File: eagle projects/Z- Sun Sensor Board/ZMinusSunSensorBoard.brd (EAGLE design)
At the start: 91 x 91 mm, 204 parts, among them J1 TE-1734829-2, U1 ADS7841E_2K5, U10 TSV991AILT, U11 TSV991AILT, U12 TSV991AILT, U13 ADS7841E_2K5, U14 TSV991AILT, U16 TSV991AILT, U17 TSV991AILT, U19 TSV991AILT, U2 ADS7841E_2K5, U21 TSV991AILT, U23 TSV991AILT, U25 ADS7841E_2K5, U26 TSV991AILT, U27 ADS7841E_2K5, U29 TSV991AILT, U3 TSV991AILT, U4 LM20BIM7X_NOPB, U5 LM20BIM7X_NOPB, U6 TSV991AILT, U8 TSV991AILT, U9 TSV991AILT

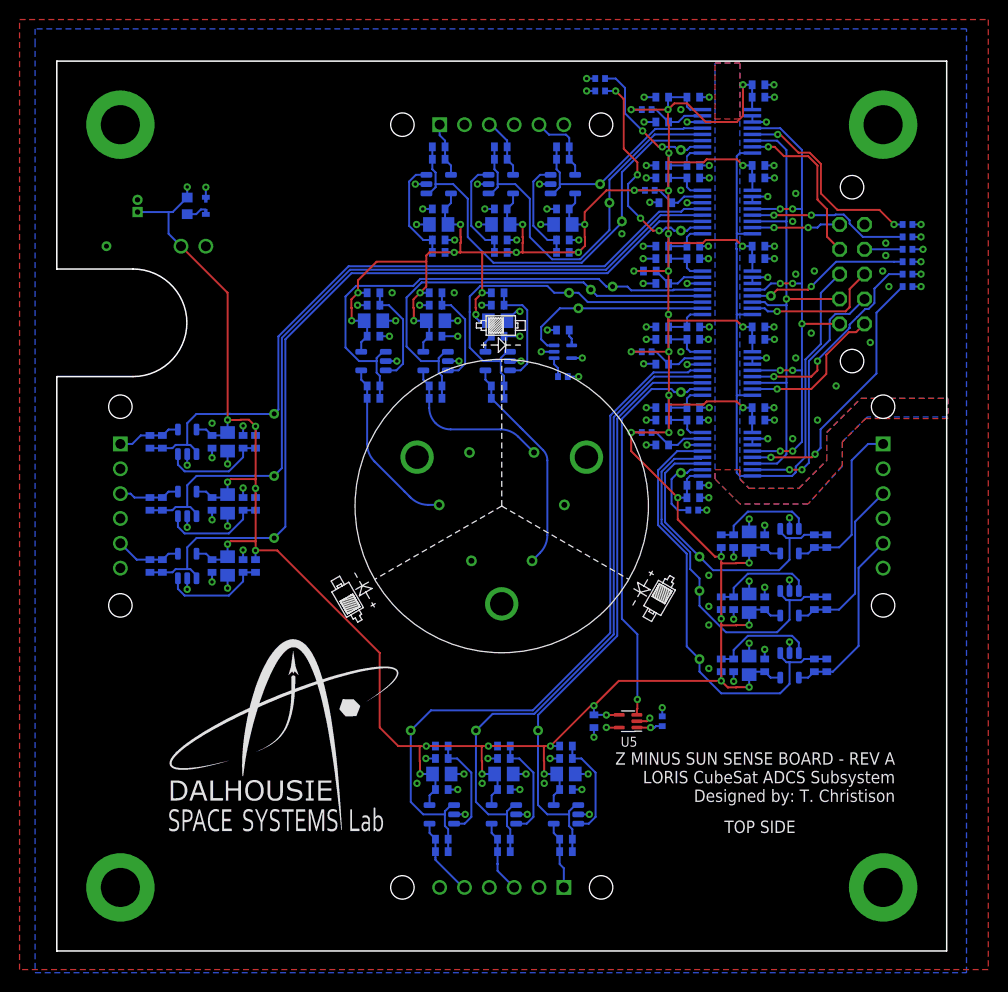
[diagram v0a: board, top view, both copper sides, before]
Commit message: I thinks its done
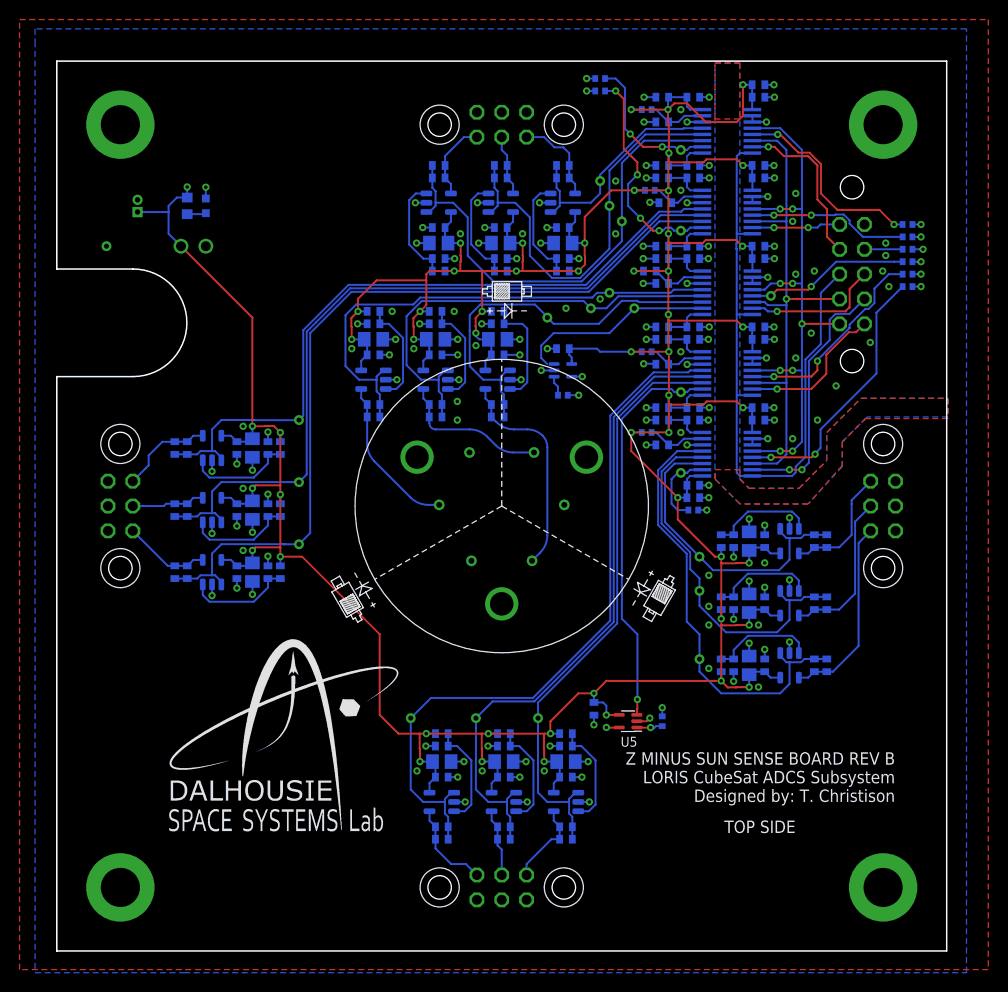
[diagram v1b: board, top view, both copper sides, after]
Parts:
- JP2, JP4, JP5, JP6: device my_library:1X06_MTG_HOLES -> my_library:2X03_MTG_HOLES
- LED1: device led:CHIPLED-0603-TTW -> led:CHIP-LED0603
- moved TP1 5.71 mm to (59.1, 65.7)
- moved U$3 3.55 mm to (46.0, 66.7)
- moved TP3 3.38 mm to (50.2, 64.8)
- moved C100 2.62 mm to (20.0, 38.7)
- moved C71 2.62 mm to (20.0, 51.4)
- moved C87 2.62 mm to (20.0, 45.1)
- moved R66 2.62 mm to (13.3, 51.4)
- moved R75 2.62 mm to (13.3, 45.1)
- moved R81 2.62 mm to (13.3, 38.7)
- moved TP23 2.62 mm to (24.8, 54.3)
- moved C101 2.62 mm to (18.4, 38.7)
- moved C103 2.62 mm to (12.1, 38.7)
- moved C82 2.62 mm to (18.4, 51.4)
- moved C83 2.62 mm to (12.1, 51.4)
- moved C88 2.62 mm to (18.4, 45.1)
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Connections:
- net GND: now also JP2.1, JP2.3, JP2.5, JP4.1, JP4.3, JP4.5, JP5.1, JP5.3, JP5.5, JP6.1, JP6.3, JP6.5, LED1.C; no longer JP2.2, JP2.4, JP2.6, JP4.2, JP4.4, JP4.6, JP5.2, JP5.4, JP5.6, JP6.2, JP6.4, JP6.6, LED1.C@1
- net N$21: now also LED1.A; no longer LED1.A@1
- net N$23: now also JP6.4; no longer JP6.3
- net N$29: now also JP6.6; no longer JP6.1
- net N$35: now also JP6.2; no longer JP6.5
- net N$37: now also JP5.2; no longer JP5.1
- net N$38: now also JP4.2; no longer JP4.1
- net N$44: now also JP4.4; no longer JP4.3
- net N$46: now also JP4.6; no longer JP4.5
- net N$49: now also JP2.2; no longer JP2.1
- net N$55: now also JP2.4; no longer JP2.3
- net N$57: now also JP2.6; no longer JP2.5
- net N$63: now also JP5.4; no longer JP5.3
- net N$65: now also JP5.6; no longer JP5.5
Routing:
- net +3V3: track 488.9 -> 497.4 mm
- net N$37: track 17.7 -> 12.5 mm
- net N$29: track 6.50 -> 9.67 mm
- net N$38: track 5.61 -> 8.14 mm
- net X-_120_DEGREES: track 40.2 -> 42.7 mm
- net X-_0_DEGREES: track 46.6 -> 49.0 mm
- net N$35: track 6.83 -> 8.89 mm
- net X-_240_DEGREES: track 22.4 -> 24.3 mm
- net N$27: track 18.0 -> 16.1 mm
- net N$63: track 18.1 -> 16.3 mm
- net N$46: track 7.68 -> 9.41 mm
- net N$49: track 6.95 -> 8.66 mm
- net Y-_120_DEGREES: track 79.6 -> 78.1 mm
- net Y-_240_DEGREES: track 74.2 -> 72.6 mm
- net N$42: track 16.8 -> 15.4 mm
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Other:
- board text added: "Z MINUS SUN SENSE BOARD REV B"
- board text removed: "Z MINUS SUN SENSE BOARD - REV A"

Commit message: done
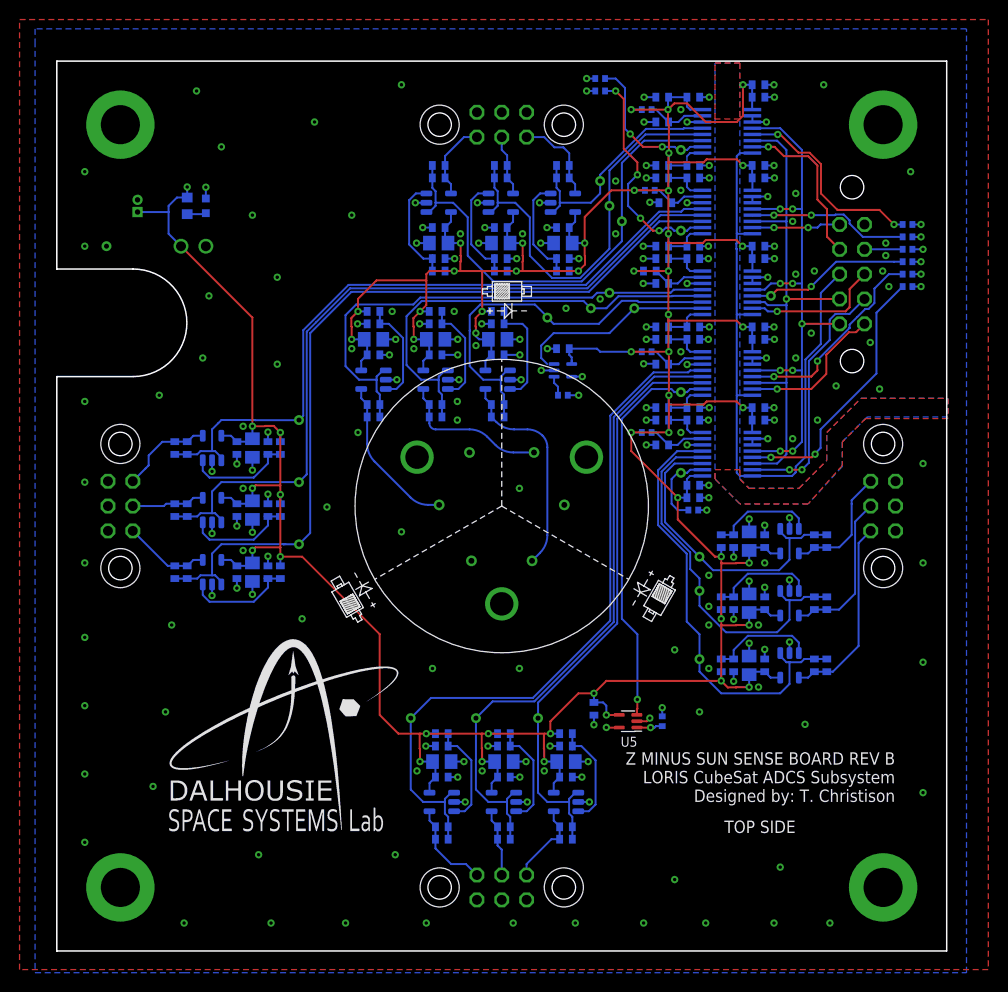
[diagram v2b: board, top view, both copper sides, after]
